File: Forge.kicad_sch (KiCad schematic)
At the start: 10 parts, among them J1 USB_C_Receptacle_USB2.0_14P, U1 ESP32-S3-WROOM-2, U2 AP2112K-3.3, U3 USBLC6-2SC6

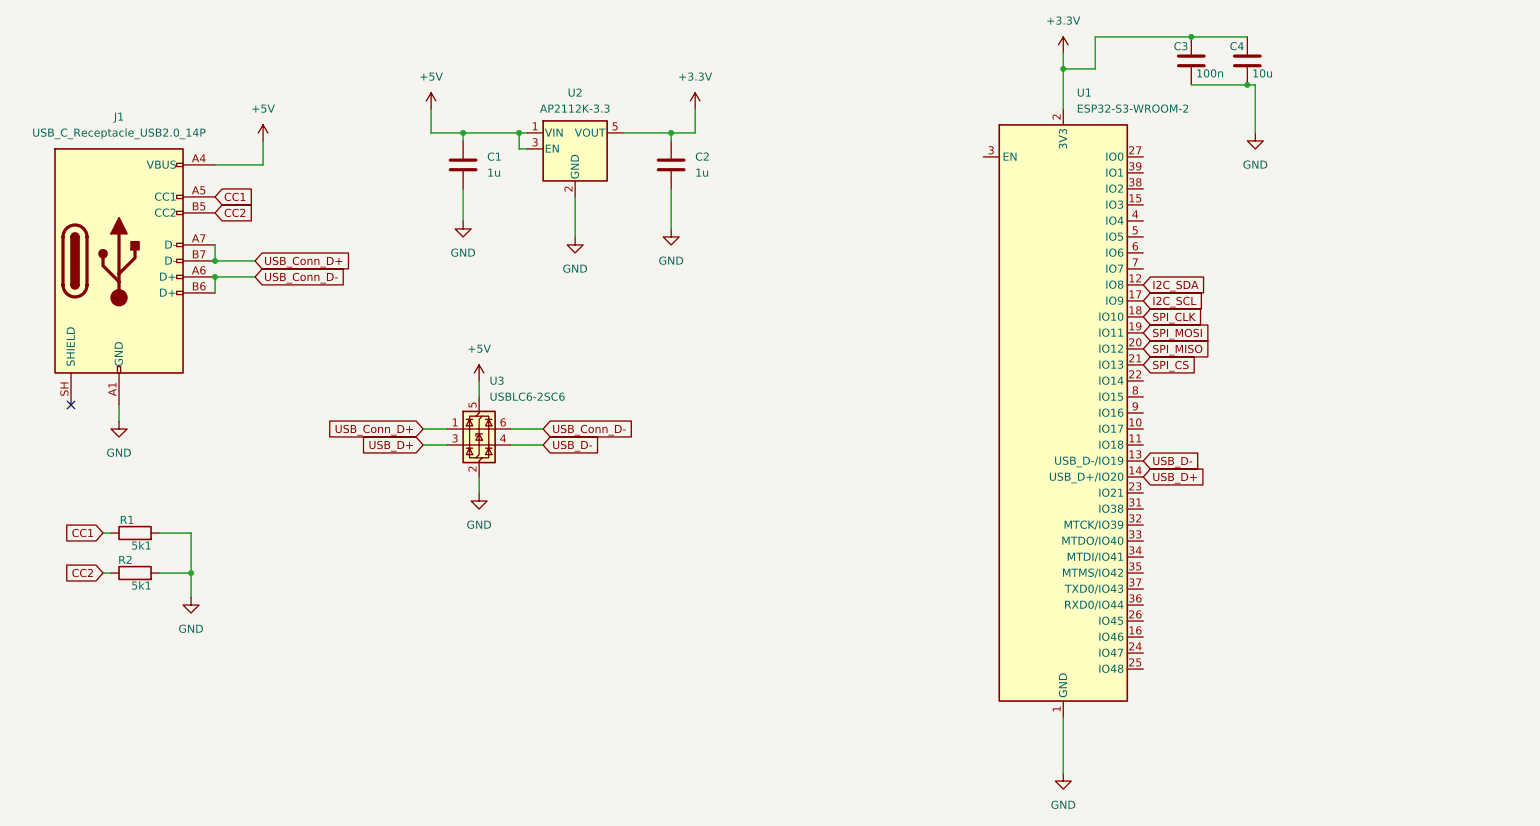
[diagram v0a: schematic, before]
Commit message: Finished schematic ready for review
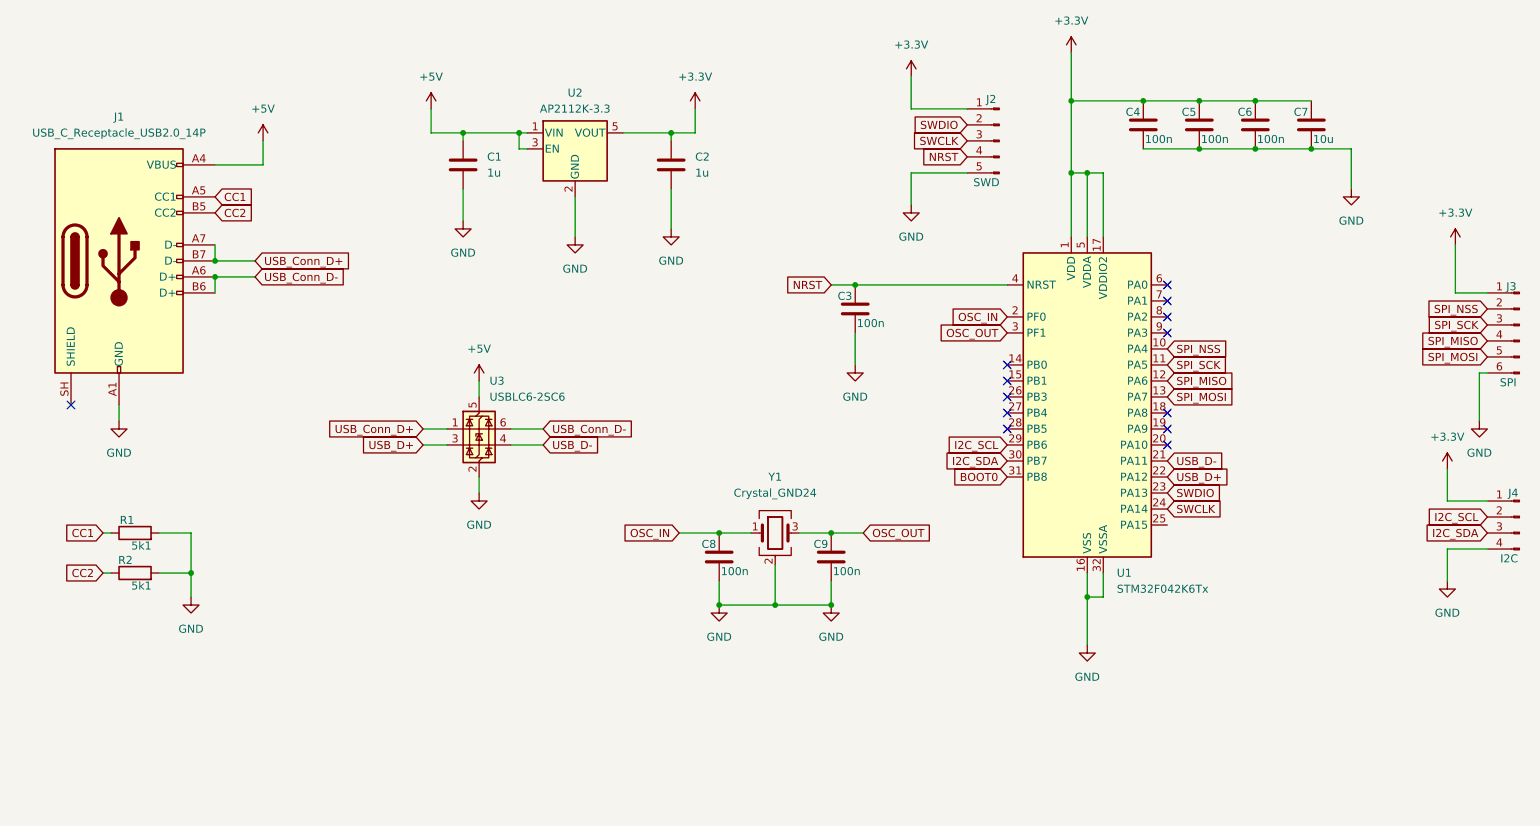
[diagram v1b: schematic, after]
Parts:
- removed U1: ESP32-S3-WROOM-2, RF_Module:ESP32-S3-WROOM-2, symbol RF_Module:ESP32-S3-WROOM-2
- added C5, C6: 100n, Capacitor_SMD:C_0805_2012Metric_Pad1.18x1.45mm_HandSolder, symbol Device:C
- added C7: 10u, Capacitor_SMD:C_0805_2012Metric_Pad1.18x1.45mm_HandSolder, symbol Device:C
- added C8, C9: 100n, Capacitor_SMD:C_0603_1608Metric_Pad1.08x0.95mm_HandSolder, symbol Device:C
- added J2: SWD, Connector_PinHeader_2.54mm:PinHeader_1x05_P2.54mm_Vertical, symbol Connector:Conn_01x05_Pin
- added J3: SPI, Connector_PinHeader_2.54mm:PinHeader_1x06_P2.54mm_Vertical, symbol Connector:Conn_01x06_Pin
- added J4: I2C, Connector_PinHeader_2.54mm:PinHeader_1x04_P2.54mm_Vertical, symbol Connector:Conn_01x04_Pin
- added U1: STM32F042K6Tx, Package_QFP:LQFP-32_7x7mm_P0.8mm, symbol MCU_ST_STM32F0:STM32F042K6Tx
- added Y1: Crystal_GND24, Crystal:Crystal_SMD_EuroQuartz_MT-4Pin_3.2x2.5mm_HandSoldering, symbol Device:Crystal_GND24
- C4: value 10u -> 100n
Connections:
- net +3.3V: now also C5.1, C6.1, C7.1, J2.1 (Pin_1), J3.1 (Pin_1), J4.1 (Pin_1), U1.1 (VDD), U1.17 (VDDIO2), U1.5 (VDDA); no longer C3.1
- net GND: now also C5.2, C6.2, C7.2, C8.2, C9.2, J2.5 (Pin_5), J3.6 (Pin_6), J4.4 (Pin_4), U1.16 (VSS), U1.32 (VSSA), Y1.2 (G), Y1.4 (G)
- net I2C_SCL: now also J4.2 (Pin_2), U1.29 (PB6)
- net I2C_SDA: now also J4.3 (Pin_3), U1.30 (PB7)
- net SPI_MISO: now also J3.4 (Pin_4), U1.12 (PA6)
- net SPI_MOSI: now also J3.5 (Pin_5), U1.13 (PA7)
- net USB_D+: now also U1.22 (PA12)
- net USB_D-: now also U1.21 (PA11)
- new net BOOT0: U1.31 (PB8)
- new net NRST: C3.1, J2.4 (Pin_4), U1.4 (NRST)
- new net OSC_IN: C8.1, U1.2 (PF0), Y1.1
- new net OSC_OUT: C9.1, U1.3 (PF1), Y1.3
- new net SPI_NSS: J3.2 (Pin_2), U1.10 (PA4)
- new net SPI_SCK: J3.3 (Pin_3), U1.11 (PA5)
- new net SWCLK: J2.3 (Pin_3), U1.24 (PA14)
- new net SWDIO: J2.2 (Pin_2), U1.23 (PA13)
- no-connect marks 1 -> 13
